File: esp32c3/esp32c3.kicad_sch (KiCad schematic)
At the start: 9 parts, among them J1 USB-C, J2 Conn_02x08_Counter_Clockwise, J3 Conn_01x01_Pin, U1 ESP32C3, U2 LM1117MP-3.3, U3 WS2812C

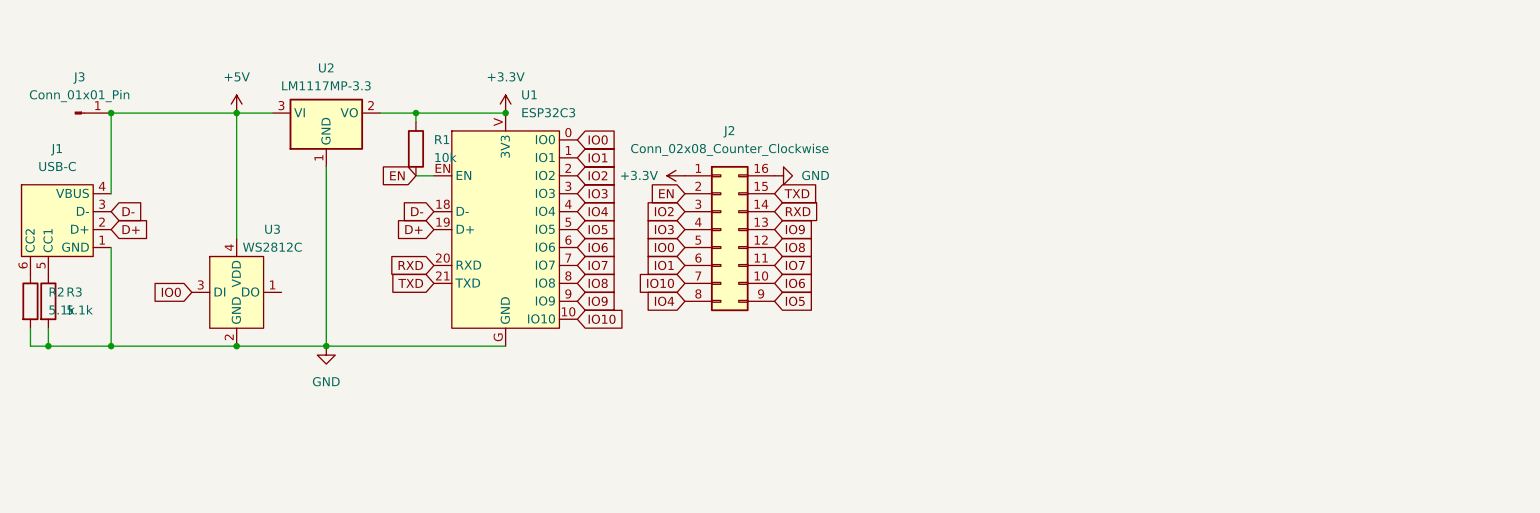
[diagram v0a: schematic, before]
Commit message: -
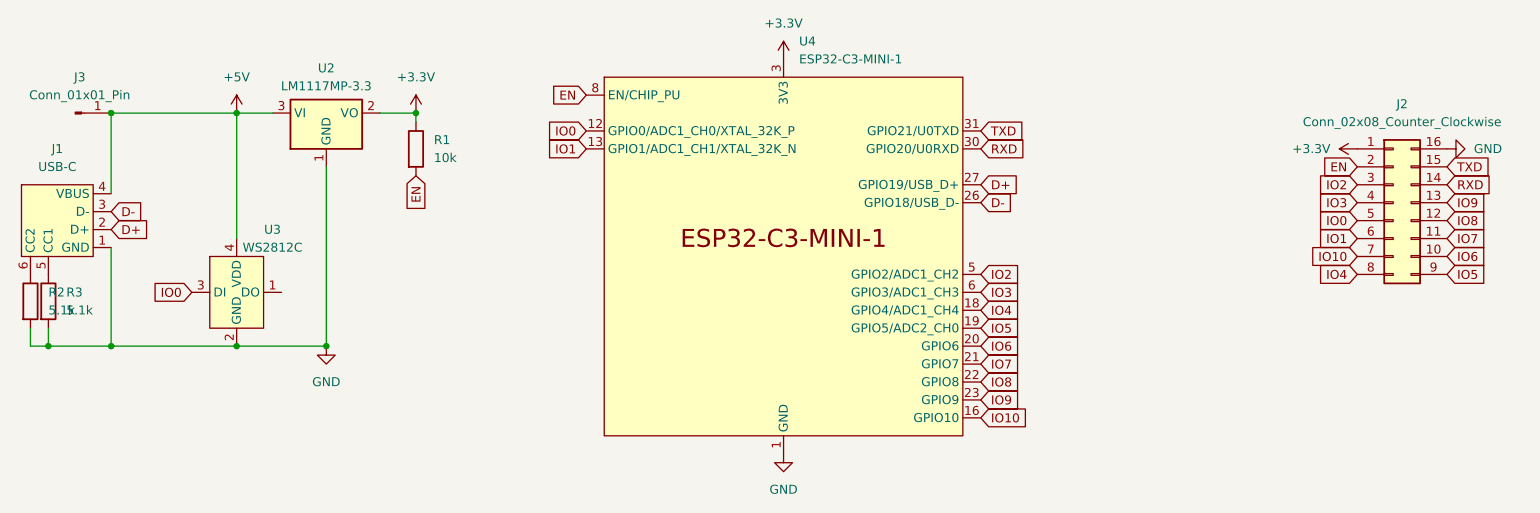
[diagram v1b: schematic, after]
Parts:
- removed U1: ESP32C3, Library:ESP32C3-MINI-1, symbol Library:ESP32C3
- added U4: ESP32-C3-MINI-1, PCM_Espressif:ESP32-C3-MINI-1, symbol Espressif:ESP32-C3-MINI-1
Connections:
- net +3.3V: now also U4.3 (3V3)
- net D+: now also U4.27 (GPIO19/USB_D+)
- net D-: now also U4.26 (GPIO18/USB_D-)
- net EN: now also U4.8 (EN/CHIP_PU)
- net GND: now also U4.1 (GND), U4.11 (GND), U4.14 (GND), U4.2 (GND), U4.36 (GND), U4.37 (GND), U4.38 (GND), U4.39 (GND), U4.40 (GND), U4.41 (GND), U4.42 (GND), U4.43 (GND), U4.44 (GND), U4.45 (GND), U4.46 (GND), U4.47 (GND), U4.48 (GND), U4.49 (GND), U4.50 (GND), U4.51 (GND), U4.52 (GND), U4.53 (GND)
- net IO0: now also U4.12 (GPIO0/ADC1_CH0/XTAL_32K_P)
- net IO1: now also U4.13 (GPIO1/ADC1_CH1/XTAL_32K_N)
- net IO10: now also U4.16 (GPIO10)
- net IO2: now also U4.5 (GPIO2/ADC1_CH2)
- net IO3: now also U4.6 (GPIO3/ADC1_CH3)
- net IO4: now also U4.18 (GPIO4/ADC1_CH4)
- net IO5: now also U4.19 (GPIO5/ADC2_CH0)
- net IO6: now also U4.20 (GPIO6)
- net IO7: now also U4.21 (GPIO7)
- net IO8: now also U4.22 (GPIO8)
- net IO9: now also U4.23 (GPIO9)
- net RXD: now also U4.30 (GPIO20/U0RXD)
- net TXD: now also U4.31 (GPIO21/U0TXD)
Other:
- moved on the sheet: J2
